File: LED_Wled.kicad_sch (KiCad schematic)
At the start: 51 parts, among them J1 SWD_PORT_SKEDD, J2 Barrel_Jack, J3 LED_VOut, J4 Microphone connector, J5 LED_signal_chan, J6 Conn_01x01, J7 5V_TP, Q1 MMBT3904, Q2 AO4485, Q3 MMBT3904, Q4 AO4485, Q5 AO4485, U1 ESP32-WROOM-32, U2 TPS5450DDAR, U3 AMS1117-3.3, U4 SN74HC125DR

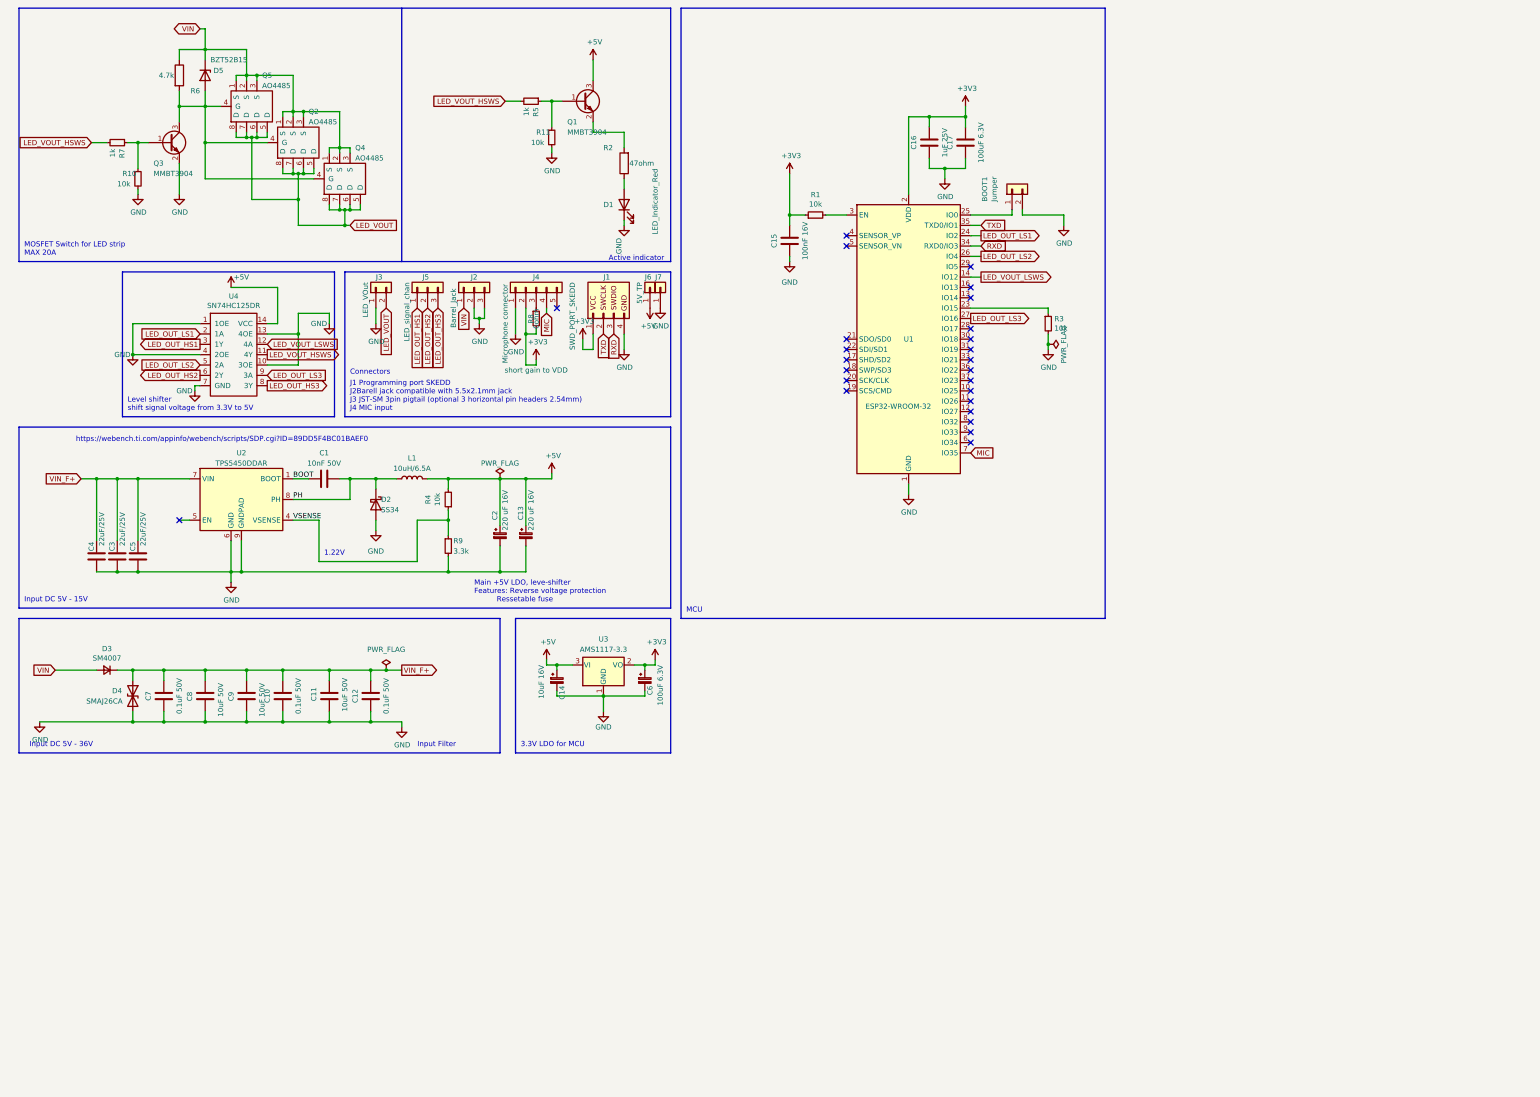
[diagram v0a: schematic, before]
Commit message: rev2.1.0 WIP
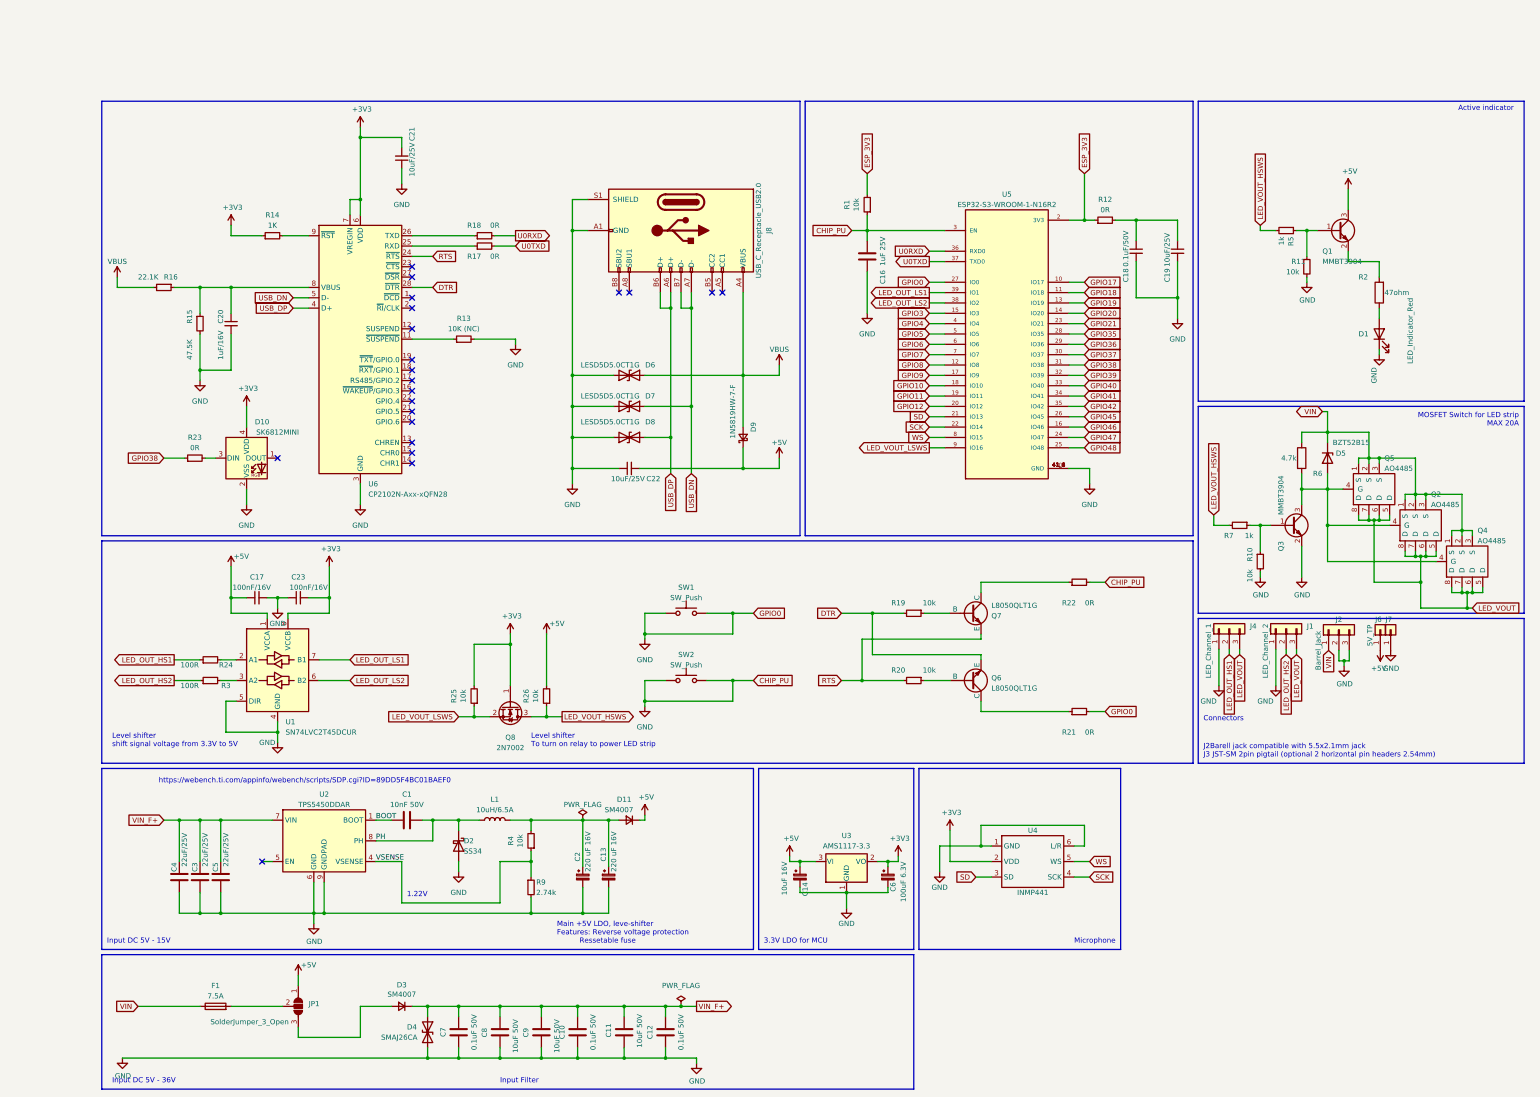
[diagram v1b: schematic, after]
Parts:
- removed BOOT1: Jumper, Connector_PinHeader_1.27mm:PinHeader_1x02_P1.27mm_Vertical, symbol Connector_Generic:Conn_01x02
- removed C15: 100nF 16V, Capacitor_SMD:C_0402_1005Metric_Pad0.74x0.62mm_HandSolder, symbol Device:C
- removed C17: 100uF 6.3V, Capacitor_SMD:C_1206_3216Metric_Pad1.33x1.80mm_HandSolder, symbol Device:C
- removed J1: SWD_PORT_SKEDD, LED_Wled:WR_WST_REDFIT_IDC_4Pin, symbol LED_Wled:SWD_PORT_SKEDD
- removed J3: LED_VOut, Connector_PinHeader_2.54mm:PinHeader_1x02_P2.54mm_Horizontal, symbol Connector_Generic:Conn_01x02
- removed J4: Microphone connector, Connector_PinSocket_2.00mm:PinSocket_1x05_P2.00mm_Vertical, symbol Connector_Generic:Conn_01x05
- removed J5: LED_signal_chan, Connector_PinHeader_2.54mm:PinHeader_1x03_P2.54mm_Horizontal, symbol Connector_Generic:Conn_01x03
- removed R8: 0ohm, Resistor_SMD:R_0805_2012Metric, symbol Device:R_Small
- removed U1: ESP32-WROOM-32, RF_Module:ESP32-WROOM-32, symbol RF_Module:ESP32-WROOM-32
- removed U4: SN74HC125DR, Package_SO:SOIC-14_3.9x8.7mm_P1.27mm, symbol LED_Wled:SN74HC125DR
- added C17, C23: 100nF/16V, symbol Device:C_Small
- added C18: 0.1uF/50V, symbol Device:C_Small
- added C19, C21, C22: 10uF/25V, symbol Device:C_Small
- added C20: 1uF/16V, symbol Device:C_Small
- added D10: SK6812MINI, LED_SMD:LED_SK6812MINI_PLCC4_3.5x3.5mm_P1.75mm, symbol LED:SK6812MINI
- added D11: SM4007, Diode_SMD:D_SOD-123F, symbol Device:D_Small
- added D6, D7, D8: LESD5D5.0CT1G, Diode_SMD:D_SOD-523, symbol Diode:ESD9B3.3ST5G
- added D9: 1N5819HW-7-F, Diode_SMD:D_SOD-123, symbol Device:D_Schottky_Small
- added F1: 7.5A, symbol Device:Fuse
- added J1: LED_Channel_2, symbol Connector_Generic:Conn_01x03
- added J4: LED_Channel_1, symbol Connector_Generic:Conn_01x03
- added J8: USB_C_Receptacle_USB2.0, symbol Connector:USB_C_Receptacle_USB2.0
- added JP1: SolderJumper_3_Open, Jumper:SolderJumper-3_P2.0mm_Open_TrianglePad1.0x1.5mm_NumberLabels, symbol Jumper:SolderJumper_3_Open
- added Q6, Q7: L8050QLT1G, Package_TO_SOT_SMD:SOT-23, symbol Simulation_SPICE:NPN
- added Q8: 2N7002, Package_TO_SOT_SMD:SOT-23, symbol Transistor_FET:2N7002
- added R12, R17, R18, R21, R22, R23: 0R, Resistor_SMD:R_0805_2012Metric, symbol Device:R_Small
- added R13: 10K (NC), Resistor_SMD:R_0805_2012Metric, symbol Device:R_Small
- added R14: 1K, Resistor_SMD:R_0805_2012Metric, symbol Device:R_Small
- added R15: 47.5K, Resistor_SMD:R_0805_2012Metric, symbol Device:R_Small
- added R16: 22.1K, Resistor_SMD:R_0805_2012Metric, symbol Device:R_Small
- added R19, R20, R25, R26: 10k, Resistor_SMD:R_0805_2012Metric, symbol Device:R_Small
- added R24: 100R, Resistor_SMD:R_0805_2012Metric, symbol Device:R_Small
- added SW1, SW2: SW_Push, symbol Switch:SW_Push
- added U1: SN74LVC2T45DCUR, Package_SO:VSSOP-8_2.4x2.1mm_P0.5mm, symbol Logic_LevelTranslator:SN74LVC2T45DCUR
- added U4: INMP441, LED_Wled:INMP441, symbol LED_Wled:INMP441
- added U5: ESP32-S3-WROOM-1-N16R2, LED_Wled:XCVR_ESP32-S3-WROOM-1-N16R2, symbol LED_Wled:ESP32-S3-WROOM-1-N16R2
- added U6: CP2102N-Axx-xQFN28, Package_DFN_QFN:QFN-28-1EP_5x5mm_P0.5mm_EP3.35x3.35mm, symbol Interface_USB:CP2102N-Axx-xQFN28
- R3: value 10k -> 100R; JLCSMT C17414 -> (none); JLCSMT_PKG 0805 -> (none); JLCSMT_Part 0805W8F1002T5E -> (none); MANUFACTURER UNI-ROYAL(Uniroyal Elec) -> (none); MFR UNI-ROYAL(Uniroyal Elec) -> (none); MPN 0805W8F1002T5E -> (none)
- R9: value 3.3k -> 2.74k; JLCSMT C22978 -> (none); JLCSMT_PKG 0603 -> (none); JLCSMT_Part 0603WAF3301T5E -> (none); MANUFACTURER UNI-ROYAL(Uniroyal Elec) -> (none); MFR UNI-ROYAL(Uniroyal Elec) -> (none)
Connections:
- net +3V3: now also C21.2, C23.2, D10.4 (VDD), Q8.1 (G), R14.1, R25.2, U1.8 (VCCB), U4.2 (VDD), U6.6 (VDD), U6.7 (VREGIN); no longer C16.2, R1.1
- net +5V: now also C17.1, C22.2, D11.1 (K), D9.1 (K), JP1.1 (A), R26.2, U1.1 (VCCA); no longer C13.1, C2.1, L1.2, R4.2
- net GND: now also C16.2, R1.1, C17.2, C18.2, C19.2, C20.2, C21.1, C22.1, C23.1, D10.2 (VSS), D6.1 (A1), D7.1 (A1), D8.1 (A1), J1.1 (Pin_1), J4.1 (Pin_1), J8.A1 (GND), J8.A12 (GND), J8.B1 (GND), J8.B12 (GND), J8.S1 (SHIELD), R13.2, R15.2, R21.2, R22.2, SW1.1, SW1.2, SW2.1, SW2.2, U1.4 (GND), U1.5 (DIR), U4.1 (GND), U4.6 (L/R), U5.1 (GND), U5.27 (IO0), U5.3 (EN), U5.40 (GND), U5.41_1 (GND), U5.41_2 (GND), U5.41_3 (GND), U5.41_4 (GND), U5.41_5 (GND), U5.41_6 (GND), U5.41_7 (GND), U5.41_8 (GND), U5.41_9 (GND), U6.29 (GND), U6.3 (GND); no longer R3.2
- net LED_OUT_HS1: now also J4.2 (Pin_2), R24.1
- net LED_OUT_HS2: now also R3.1, J1.2 (Pin_2)
- net LED_OUT_LS1: now also U1.7 (B1), U5.39 (IO1)
- net LED_OUT_LS2: now also U1.6 (B2), U5.38 (IO2)
- net LED_VOUT: now also J1.3 (Pin_3), J4.3 (Pin_3)
- net LED_VOUT_HSWS: now also Q8.3 (D), R26.1
- net LED_VOUT_LSWS: now also Q8.2 (S), R25.1, U5.9 (IO16)
- net VIN: now also F1.1; no longer D3.2 (A)
- net ESP_3V3: now reaches R1.2
- net ESP_3V3: now also R12.1, U5.2 (3V3)
- new net: C13.1, C2.1, D11.2 (A), L1.2, R4.2
- new net: D3.2 (A), JP1.3 (B)
- new net: Q7.2 (B), R19.1
- new net: R14.2, U6.9 (~{RST})
- new net: R3.2, U1.3 (A2)
- new net: Q6.2 (B), R20.1
- new net: Q7.1 (C), R22.1
- new net: C20.1, R15.1, R16.1, U6.8 (VBUS)
- new net: R17.1, U6.26 (TXD)
- new net: C18.1, C19.1, R12.2
- new net: R24.2, U1.2 (A1)
- new net: F1.2, JP1.2 (C)
- new net: R13.1, U6.11 (~{SUSPEND})
- new net: R18.1, U6.25 (RXD)
- new net: Q6.1 (C), R21.1
- new net: D10.3 (DIN), R23.2
- new net DTR: Q6.3 (E), R19.2, U6.28 (~{DTR})
- new net GPIO10: U5.18 (IO10)
- new net GPIO11: U5.19 (IO11)
- new net GPIO12: U5.20 (IO12)
- new net GPIO17: U5.10 (IO17)
- new net GPIO18: U5.11 (IO18)
- new net GPIO19: U5.13 (IO19)
- new net GPIO20: U5.14 (IO20)
- new net GPIO21: U5.23 (IO21)
- new net GPIO3: U5.15 (IO3)
- new net GPIO35: U5.28 (IO35)
- new net GPIO36: U5.29 (IO36)
- new net GPIO37: U5.30 (IO37)
- new net GPIO38: R23.1, U5.31 (IO38)
- new net GPIO39: U5.32 (IO39)
- new net GPIO4: U5.4 (IO4)
- new net GPIO40: U5.33 (IO40)
- new net GPIO41: U5.34 (IO41)
- new net GPIO42: U5.35 (IO42)
- new net GPIO45: U5.26 (IO45)
- new net GPIO46: U5.16 (IO46)
- new net GPIO47: U5.24 (IO47)
- new net GPIO48: U5.25 (IO48)
- new net GPIO5: U5.5 (IO5)
- new net GPIO6: U5.6 (IO6)
- new net GPIO7: U5.7 (IO7)
- new net GPIO8: U5.12 (IO8)
- new net GPIO9: U5.17 (IO9)
- new net RTS: Q7.3 (E), R20.2, U6.24 (~{RTS})
- new net SCK: U4.4 (SCK), U5.22 (IO14)
- new net SD: U4.3 (SD), U5.21 (IO13)
- new net U0RXD: R17.2, U5.36 (RXD0)
- new net U0TXD: R18.2, U5.37 (TXD0)
- new net USB_DN: D7.2 (A2), J8.A7 (D-), J8.B7 (D-), U6.5 (D-)
- new net USB_DP: D8.2 (A2), J8.A6 (D+), J8.B6 (D+), U6.4 (D+)
- new net VBUS: D6.2 (A2), D9.2 (A), J8.A4 (VBUS), J8.A9 (VBUS), J8.B4 (VBUS), J8.B9 (VBUS), R16.2
- new net WS: U4.5 (WS), U5.8 (IO15)
- no-connect marks 25 -> 21
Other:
- note added: "J2Barell jack compatible with 5.5x2.1mm jack J3 JST-SM 2pin pigtail (optional 2 horizontal pin headers 2.54mm)"
- note added: "Level shifter To turn on relay to power LED strip"
- note added: "Microphone"
- note removed: "J1 Programming port SKEDD J2Barell jack compatible with 5.5x2.1mm jack J3 JST-SM 3pin pigtail (optional 3 horizontal pin headers 2.54mm) J4 MIC input"
- note removed: "MCU"
- moved on the sheet: C1, C10, C11, C12, C13, C14, C16, C2, C3, C4, C5, C6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
